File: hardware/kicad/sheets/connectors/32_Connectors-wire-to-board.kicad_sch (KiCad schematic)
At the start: 46 parts

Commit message: imrpved footprints
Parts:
- -12V+_4, -12V+_5, -12V+_6: footprint 5v rail sm-easyedapro:CONN-TH_2P-P3.96_VH3.96-2AW -> Connector_JST:JST_VH_B2P-VH_1x02_P3.96mm_Vertical
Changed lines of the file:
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@@
 			)
 		)
-		(property "Footprint" "5v rail sm-easyedapro:CONN-TH_2P-P3.96_VH3.96-2AW"
+		(property "Footprint" "Connector_JST:JST_VH_B2P-VH_1x02_P3.96mm_Vertical"
 			(at 363.22 149.86 0)
 			(effects
@@
 			)
 		)
-		(property "Footprint" "5v rail sm-easyedapro:CONN-TH_2P-P3.96_VH3.96-2AW"
+		(property "Footprint" "Connector_JST:JST_VH_B2P-VH_1x02_P3.96mm_Vertical"
 			(at 22.86 165.1 0)
 			(effects
@@
 			)
 		)
-		(property "Footprint" "5v rail sm-easyedapro:CONN-TH_2P-P3.96_VH3.96-2AW"
+		(property "Footprint" "Connector_JST:JST_VH_B2P-VH_1x02_P3.96mm_Vertical"
 			(at 284.48 106.68 0)
 			(effects

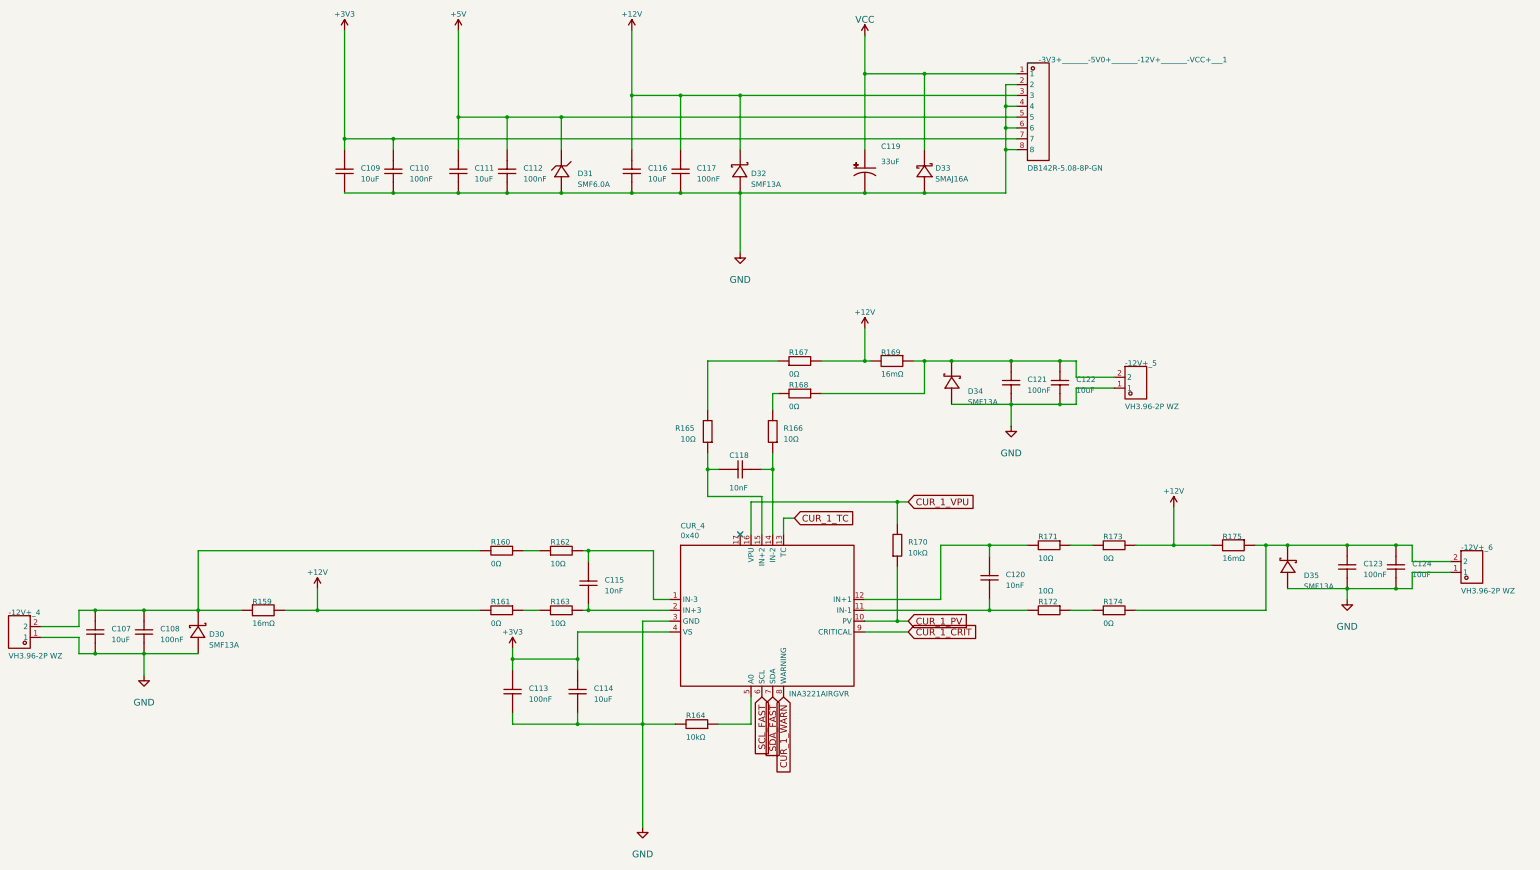
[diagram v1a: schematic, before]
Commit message: added better footprints and steps
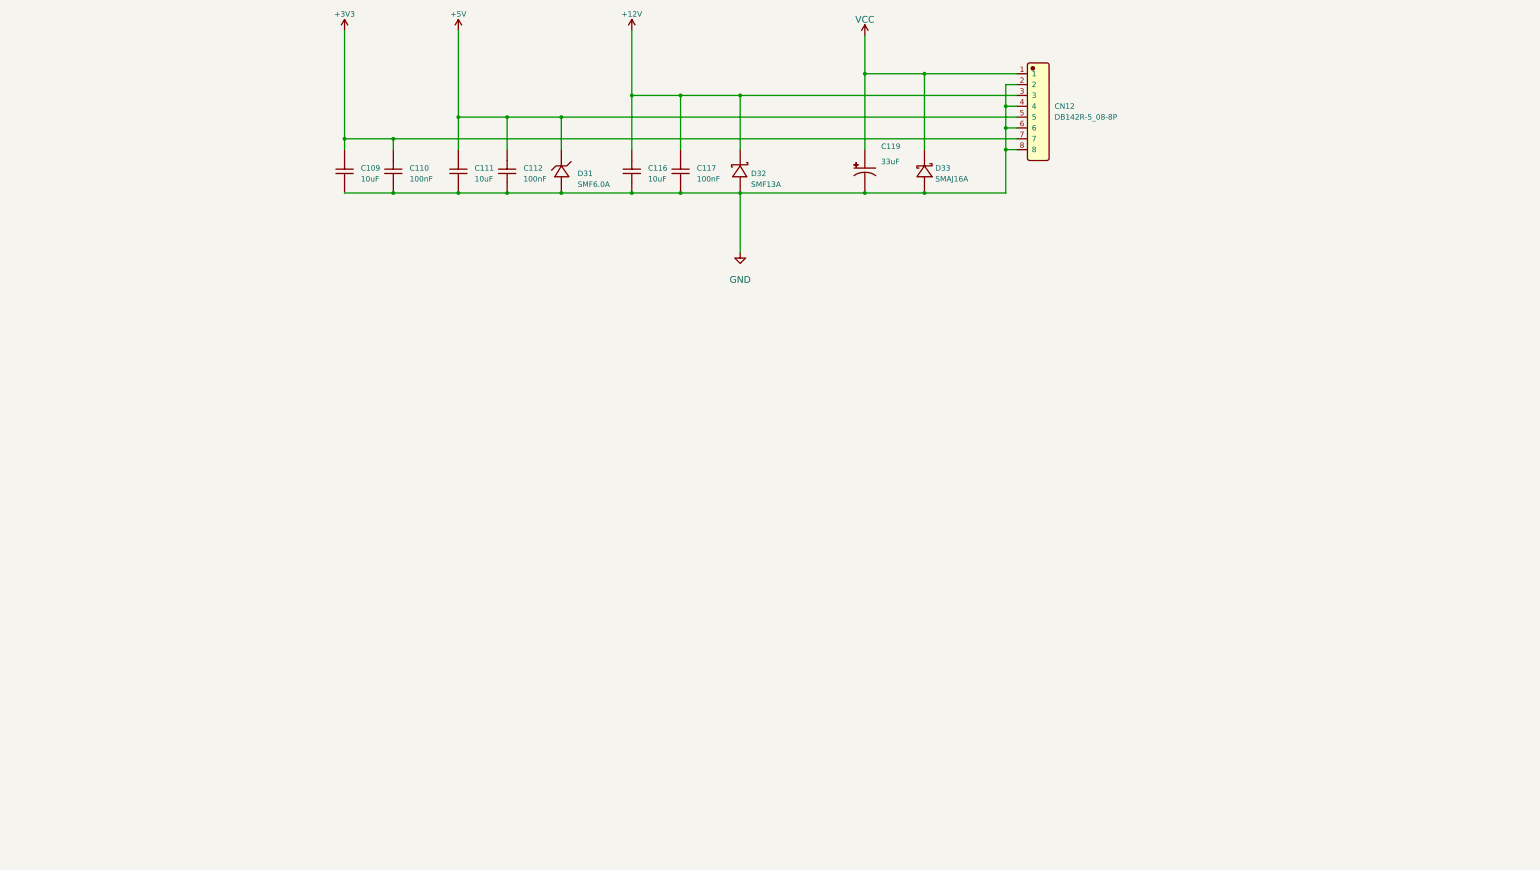
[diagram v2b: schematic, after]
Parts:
- removed -12V+_4, -12V+_5, -12V+_6: VH3.96-2P WZ, Connector_JST:JST_VH_B2P-VH_1x02_P3.96mm_Vertical, symbol 5v rail sm-easyedapro:VH3.96-2P WZ
- removed C107, C114, C122, C124: 10uF, Capacitor_SMD:C_0805_2012Metric, symbol 5v rail sm-easyedapro:GRM21BR61H106KE43L
- removed C108, C113, C121, C123: 100nF, Capacitor_SMD:C_0603_1608Metric, symbol 5v rail sm-easyedapro:CC0603KRX7R9BB104
- removed C115, C118, C120: 10nF, Capacitor_SMD:C_0201_0603Metric, symbol 5v rail sm-easyedapro:TCC0201X7R103K500ZT
- removed CUR_4: INA3221AIRGVR, Package_DFN_QFN:QFN-16-1EP_4x4mm_P0.65mm_EP2.2x2.2mm, symbol 5v rail sm-easyedapro:INA3221AIRGVR
- removed D30, D34, D35: SMF13A, Diode_SMD:SOD-123FL, symbol 5v rail sm-easyedapro:SMF13A_C353315
- removed R159, R169, R175: 16mΩ, Resistor_SMD:R_2512_6332Metric, symbol 5v rail sm-easyedapro:LR123WF160MT4E
- removed R160, R161, R167, R168, R173, R174: 0Ω, Resistor_SMD:R_0201_0603Metric, symbol 5v rail sm-easyedapro:RC0201FR-070RL
- removed R162, R163, R165, R166, R171, R172: 10Ω, Resistor_SMD:R_0402_1005Metric, symbol 5v rail sm-easyedapro:RC0402FR-0710RL
- removed R164, R170: 10kΩ, Resistor_SMD:R_0402_1005Metric, symbol 5v rail sm-easyedapro:0402WGF1002TCE
- removed ___-3V3+_______-5V0+_______-12V+_______-VCC+___1: DB142R-5.08-8P-GN, 5v rail sm-easyedapro:CONN-TH_8P-P5.08_DIBO_DB142R-5.08-8P, symbol 5v rail sm-easyedapro:DB142R-5.08-8P
- added CN12: DB142R-5_08-8P, JLCImport:DB142R-5_08-8P, symbol JLCImport:DB142R-5_08-8P
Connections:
- net +12V: now also CN12.3
- net +3V3: now also CN12.7
- net +5V: now also CN12.5
- net GND: now also CN12.2, CN12.4, CN12.6, CN12.8
- net VCC: now also CN12.1
- no-connect marks 1 -> 0
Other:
- note removed: "0x40"
